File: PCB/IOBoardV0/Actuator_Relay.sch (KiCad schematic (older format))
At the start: 15 parts, among them J1 RJ45_2, J2 RJ45_2, K1 RELAY_J9906, P1 KLEMENS_1, P2 CONN_8X2, Q1 BC557, Q2 2N2222A

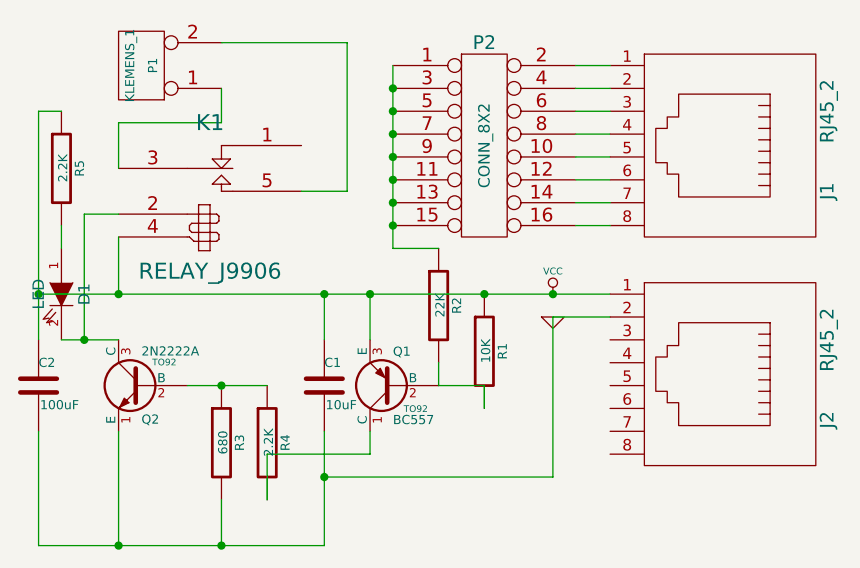
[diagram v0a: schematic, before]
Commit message: Add files via upload
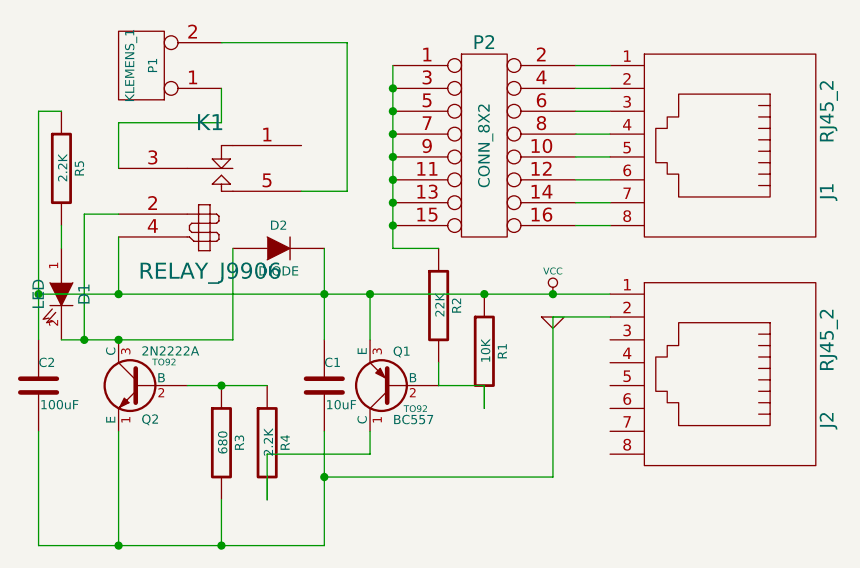
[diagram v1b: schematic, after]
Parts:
- added D2: DIODE, ~, symbol DIODE
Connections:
- net VCC: now also D2.2 (K)
- net at D1.2 (K), K1.2 (COIL1), Q2.3 (C): now also D2.1 (A)
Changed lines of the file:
@@
 Sheet 1 1
 Title "noname.sch"
-Date "23 apr 2020"
+Date "28 jun 2020"
 Rev ""
 Comp ""
@@
 	2600 2250 2600 2150
 Wire Wire Line
-	2100 2050 2100 1850
+	2100 1650 2100 2050
 Connection ~ 2800 1850
 Wire Wire Line
@@
 	1050 1500 1050 2050
 Wire Wire Line
-	950  2050 1200 2050
+	950  2050 1700 2050
 $Comp
 L R R5
@@
 Wire Wire Line
 	1650 1100 1650 950
+$Comp
+L DIODE D2
+U 1 1 5EF8356A
+P 1900 1650
+F 0 "D2" H 1900 1750 40  0000 C CNN
+F 1 "DIODE" H 1900 1550 40  0000 C CNN
+F 2 "~" H 1900 1650 60  0000 C CNN
+F 3 "~" H 1900 1650 60  0000 C CNN
+	1    1900 1650
+	1    0    0    -1
+$EndComp
+Wire Wire Line
+	1700 2050 1700 1650
+Connection ~ 1200 2050
 $EndSCHEMATC
